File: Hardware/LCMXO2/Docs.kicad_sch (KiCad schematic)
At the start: 0 parts

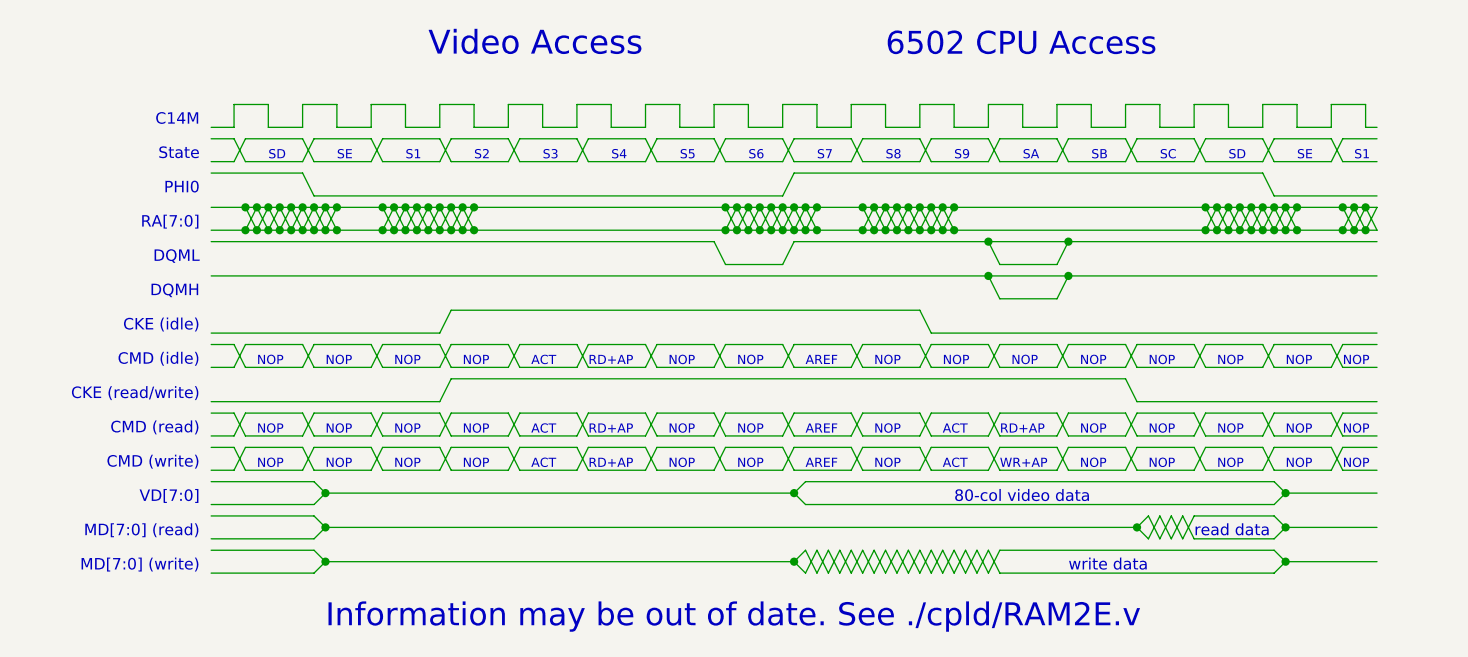
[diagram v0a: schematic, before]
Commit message: As sent to testers
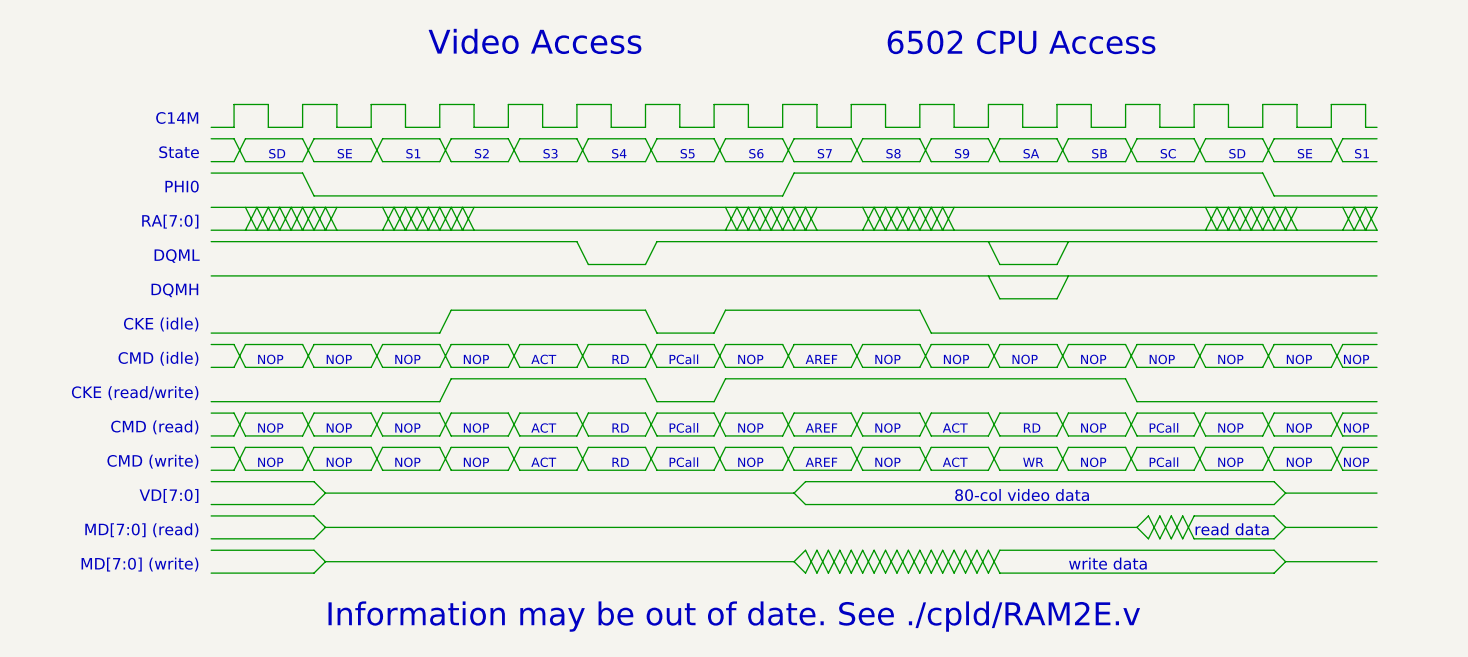
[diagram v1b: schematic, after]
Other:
- note added: "PCall"
- note added: "RD"
- note added: "WR"
- note removed: "RD+AP"
- note removed: "WR+AP"
